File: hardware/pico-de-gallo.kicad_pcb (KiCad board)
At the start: 2 copper layers, 50 x 69.5 mm, 9 parts, among them J1 Conn_01x04_Socket, J2 Conn_01x05_Socket, J3 Conn_01x08_Pin

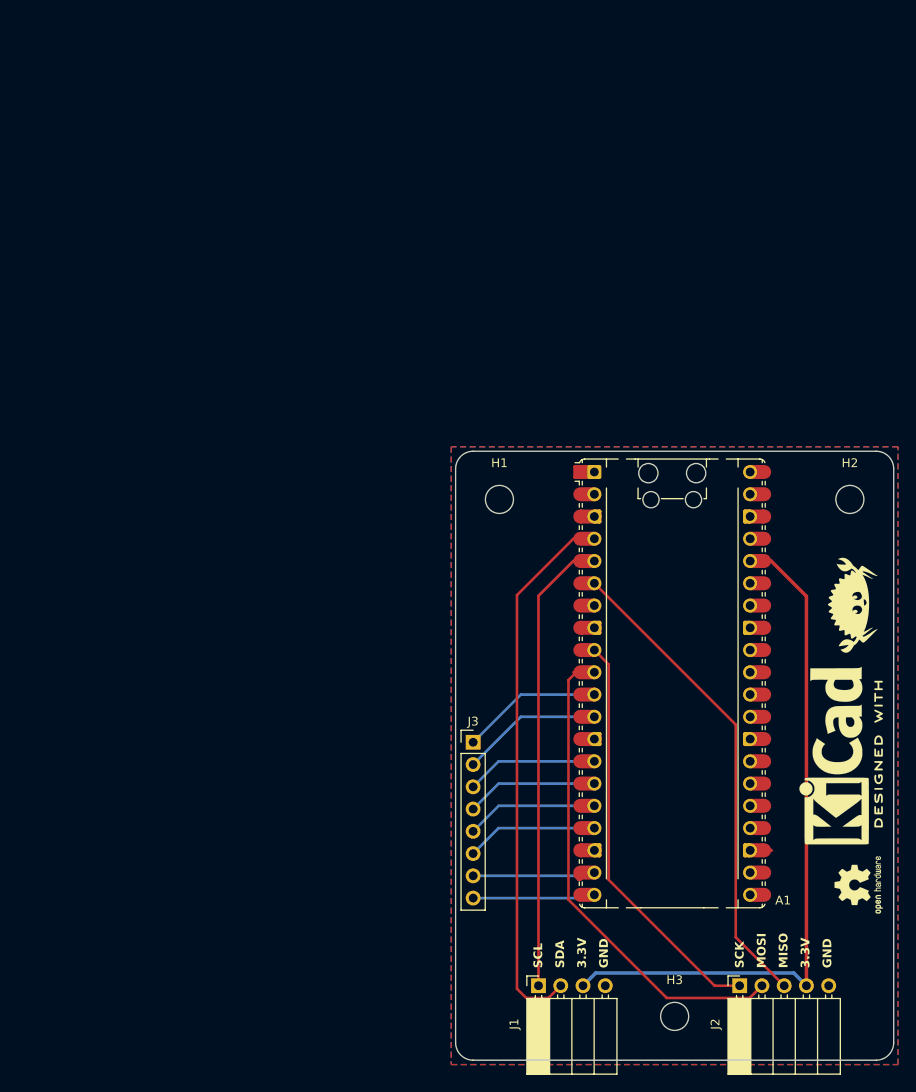
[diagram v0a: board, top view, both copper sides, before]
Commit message: update case and PCB
Signed-off-by: Felipe Balbi <febalbi@microsoft.com>
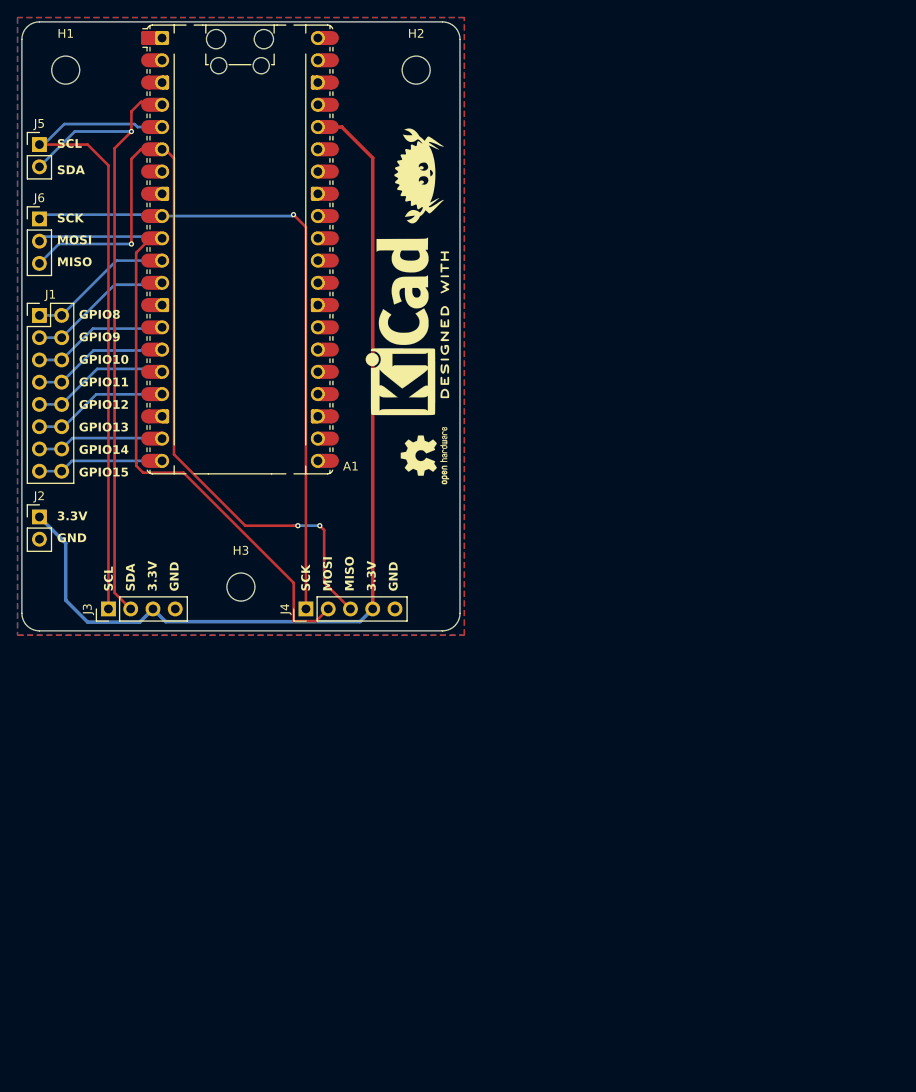
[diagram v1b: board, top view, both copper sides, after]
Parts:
- added J4: Conn_01x05, Connector_PinHeader_2.54mm:PinHeader_1x05_P2.54mm_Vertical, F.Cu at (32.9, 67.5)
- added J5: Conn_01x02, Connector_PinHeader_2.54mm:PinHeader_1x02_P2.54mm_Vertical, F.Cu at (2.50, 14.5)
- added J6: Conn_01x03, Connector_PinHeader_2.54mm:PinHeader_1x03_P2.54mm_Vertical, F.Cu at (2.50, 23.0)
- J1: value Conn_01x04_Socket -> Conn_02x08_Odd_Even; footprint Connector_PinSocket_2.54mm:PinSocket_1x04_P2.54mm_Horizontal -> Connector_PinHeader_2.54mm:PinHeader_2x08_P2.54mm_Vertical
- J2: value Conn_01x05_Socket -> Conn_01x02; footprint Connector_PinSocket_2.54mm:PinSocket_1x05_P2.54mm_Horizontal -> Connector_PinHeader_2.54mm:PinHeader_1x02_P2.54mm_Vertical
- J3: value Conn_01x08_Pin -> Conn_01x04; footprint Connector_PinHeader_2.54mm:PinHeader_1x08_P2.54mm_Vertical -> Connector_PinHeader_2.54mm:PinHeader_1x04_P2.54mm_Vertical
- moved J2 96.2 mm to (2.50, 57.0), turned to 0 degrees
- moved J1 95.4 mm to (2.50, 34.0), turned to 0 degrees
- moved A1 69.9 mm to (25.4, 26.5)
- moved H1 69.7 mm to (5.50, 6.00)
- moved H2 69.7 mm to (45.5, 6.00)
- moved H3 69.7 mm to (25.5, 65.0)
- moved REF** 69.7 mm to (43.7, 35.2)
- moved REF** 69.7 mm to (46.5, 50.0)
- moved J3 44.3 mm to (10.4, 67.5), turned to 90 degrees
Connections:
- J1 pad 1: /SCL -> /GPIO8
- J1 pad 2: /SDA -> /GPIO8
- J1 pad 3: +3V3 -> /GPIO9
- J1 pad 4: GND -> /GPIO9
- J2 pad 1: /CLK -> +3V3
- J2 pad 2: /MOSI -> GND
- J3 pad 1: /GPIO8 -> /SCL
- J3 pad 2: /GPIO9 -> /SDA
- J3 pad 3: /GPIO10 -> +3V3
- J3 pad 4: /GPIO11 -> GND
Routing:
- net /MISO: track 54.9 -> 92.8 mm, vias 0 -> 3
- net +3V3: track 78.4 -> 107.0 mm
- net /CLK: track 46.9 -> 74.9 mm, vias 0 -> 1
- net /SCL: track 51.7 -> 74.3 mm
- net /MOSI: track 57.3 -> 74.5 mm
- net /SDA: track 61.6 -> 73.7 mm, vias 0 -> 1
- net GND: track 1.60 -> 0.00 mm
- net /GPIO14: track 16.0 -> 14.6 mm
- net /GPIO13: track 15.0 -> 15.7 mm
- net /GPIO8: track 16.1 -> 16.7 mm
- net /GPIO10: track 15.0 -> 15.7 mm
- net /GPIO9: track 16.1 -> 16.7 mm
- net /GPIO12: track 15.0 -> 15.7 mm
- net /GPIO11: track 15.0 -> 15.7 mm
- net /GPIO15: track 14.0 -> 14.6 mm
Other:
- board text added: "Felipe Balbi - 2025"
- board text added: "GPIO10"
- board text added: "GPIO11"
- board text added: "GPIO12"
- board text added: "GPIO13"
- board text added: "GPIO14"
- board text added: "GPIO15"
- board text added: "GPIO8"
- board text added: "GPIO9"
